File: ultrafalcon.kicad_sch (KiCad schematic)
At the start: 1 part, among them SW1 RotaryEncoder

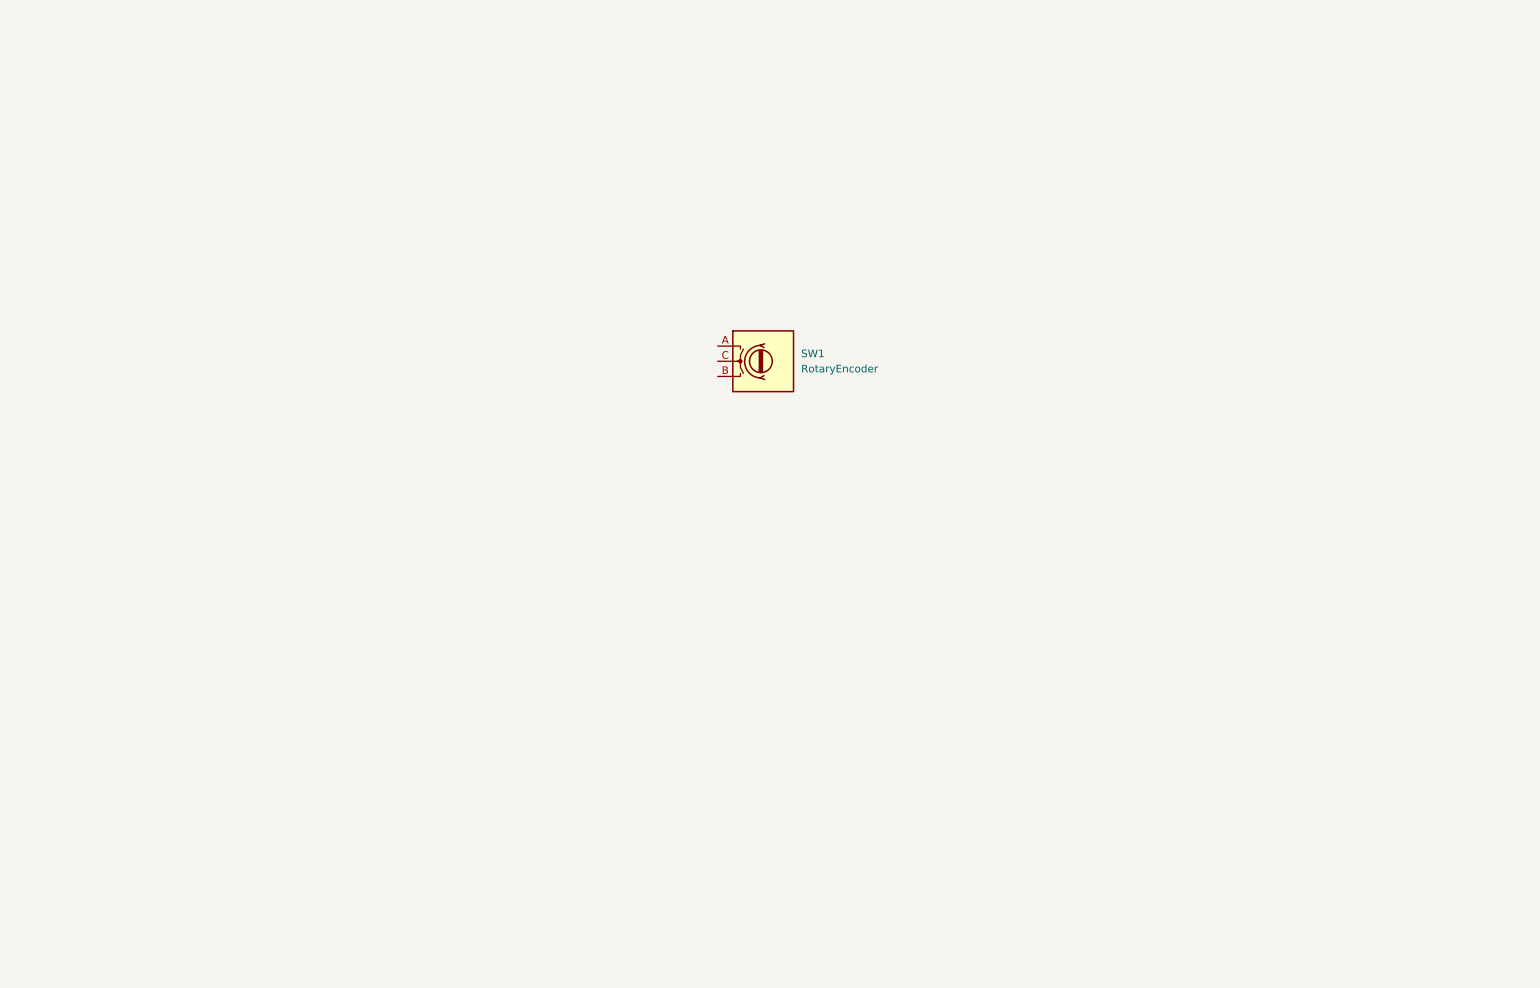
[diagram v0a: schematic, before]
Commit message: jan17 updates
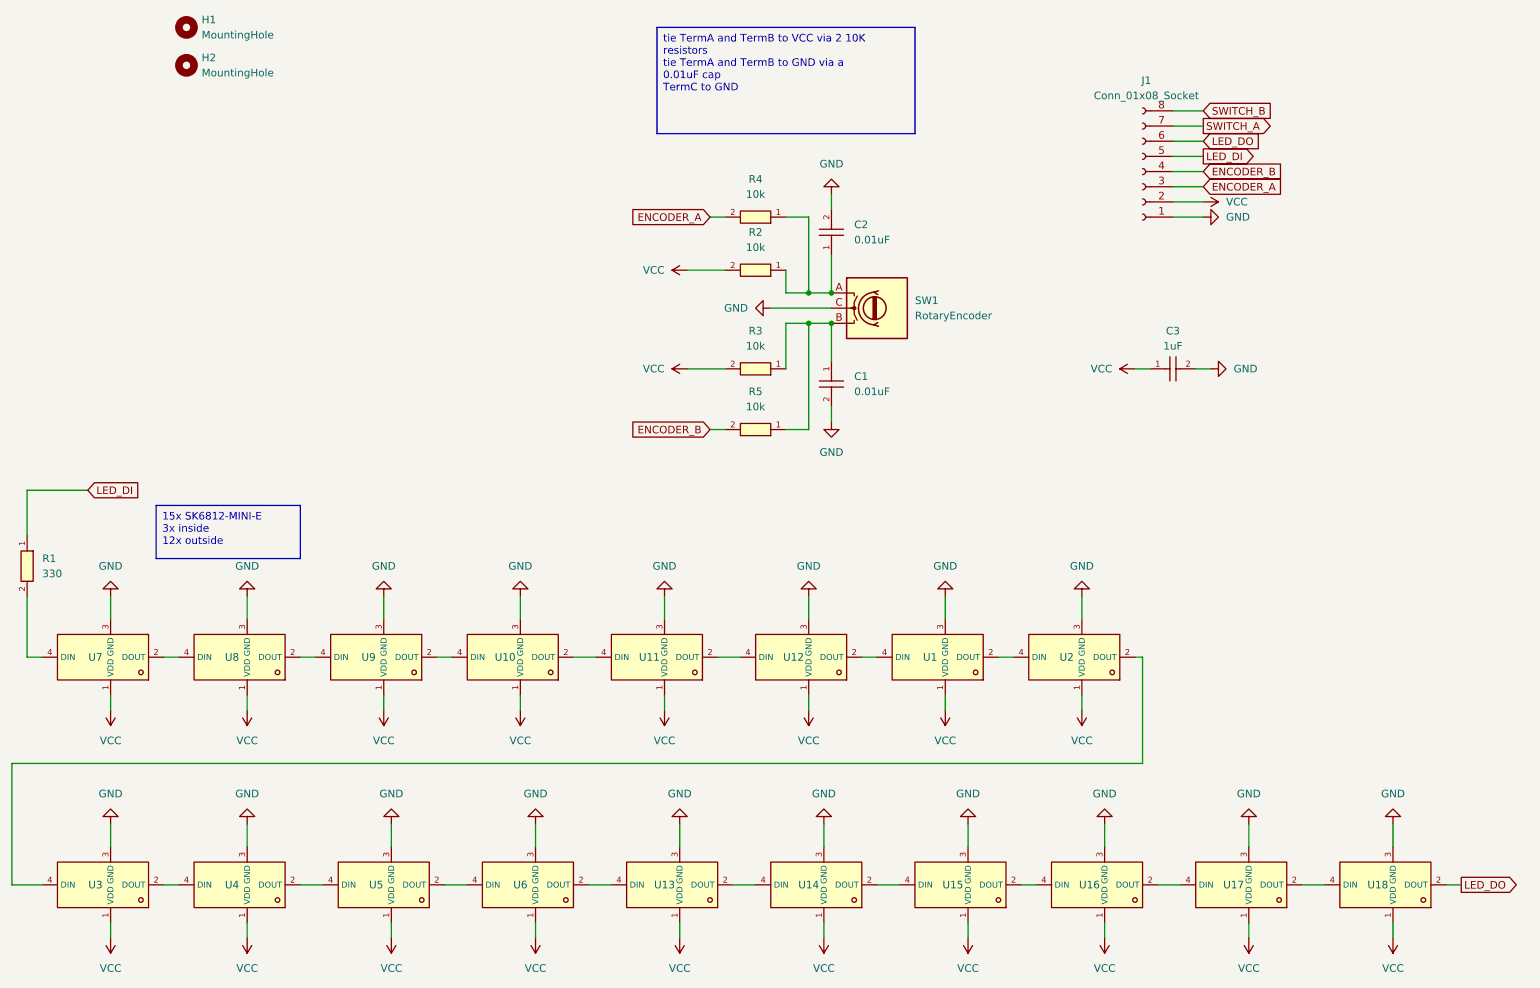
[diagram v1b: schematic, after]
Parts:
- added C1, C2: 0.01uF, ct-kicad:C0402, symbol ct-kicad:CL05B104KO5NNNC
- added C3: 1uF, ct-kicad:C0402, symbol ct-kicad:CL05B104KO5NNNC
- added H1, H2: MountingHole, MountingHole:MountingHole_3.2mm_M3_Pad_Via, symbol Mechanical:MountingHole
- added J1: Conn_01x08_Socket, Connector_JST:JST_EH_B8B-EH-A_1x08_P2.50mm_Vertical, symbol Connector:Conn_01x08_Socket
- added R1: 330, ct-kicad:R0603, symbol ct-kicad:0603WAF3300T5E
- added R2, R3, R4, R5: 10k, ct-kicad:R0603, symbol ct-kicad:0603WAF3300T5E
- added U1, U10, U11, U12, U13, U14, U15, U16, U17, U18, U2, U3, U4, U5, U6, U7, U8, U9: SK6812MINI-E_C5149201, ct-kicad:YS-SK6812MINI-E-casuanoob, symbol ct-kicad:SK6812MINI-E_C5149201
- SW1: footprint fingerpunch:PERS56v3 -> ct-kicad:PER60
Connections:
- net at SW1.A: now also C2.1, R2.1, R4.1
- net at SW1.B: now also C1.1, R3.1, R5.1
- net GND: now reaches SW1.C
- net GND: now also C1.2, C2.2, C3.2, J1.1 (Pin_1), U1.3 (GND), U10.3 (GND), U11.3 (GND), U12.3 (GND), U13.3 (GND), U14.3 (GND), U15.3 (GND), U16.3 (GND), U17.3 (GND), U18.3 (GND), U2.3 (GND), U3.3 (GND), U4.3 (GND), U5.3 (GND), U6.3 (GND), U7.3 (GND), U8.3 (GND), U9.3 (GND)
- new net: U15.2 (DOUT), U16.4 (DIN)
- new net: U14.2 (DOUT), U15.4 (DIN)
- new net: U13.4 (DIN), U6.2 (DOUT)
- new net: U5.2 (DOUT), U6.4 (DIN)
- new net: U11.2 (DOUT), U12.4 (DIN)
- new net: U10.2 (DOUT), U11.4 (DIN)
- new net: R1.2, U7.4 (DIN)
- new net: U4.2 (DOUT), U5.4 (DIN)
- new net: U3.2 (DOUT), U4.4 (DIN)
- new net: U16.2 (DOUT), U17.4 (DIN)
- new net: U2.2 (DOUT), U3.4 (DIN)
- new net: U17.2 (DOUT), U18.4 (DIN)
- new net: U8.2 (DOUT), U9.4 (DIN)
- new net: U7.2 (DOUT), U8.4 (DIN)
- new net: U10.4 (DIN), U9.2 (DOUT)
- new net: U13.2 (DOUT), U14.4 (DIN)
- new net: U1.4 (DIN), U12.2 (DOUT)
- new net: U1.2 (DOUT), U2.4 (DIN)
- new net ENCODER_A: J1.3 (Pin_3), R4.2
- new net ENCODER_B: J1.4 (Pin_4), R5.2
- new net LED_DI: J1.5 (Pin_5), R1.1
- new net LED_DO: J1.6 (Pin_6), U18.2 (DOUT)
- new net SWITCH_A: J1.7 (Pin_7)
- new net SWITCH_B: J1.8 (Pin_8)
- new net VCC: C3.1, J1.2 (Pin_2), R2.2, R3.2, U1.1 (VDD), U10.1 (VDD), U11.1 (VDD), U12.1 (VDD), U13.1 (VDD), U14.1 (VDD), U15.1 (VDD), U16.1 (VDD), U17.1 (VDD), U18.1 (VDD), U2.1 (VDD), U3.1 (VDD), U4.1 (VDD), U5.1 (VDD), U6.1 (VDD), U7.1 (VDD), U8.1 (VDD), U9.1 (VDD)
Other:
- moved on the sheet: SW1
